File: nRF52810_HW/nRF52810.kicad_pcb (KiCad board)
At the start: 4 copper layers, 62.2 x 65.2 mm, 70 parts, among them J1 TC2050-IDC-NL, Q1 BSS138PW,115, U1 NRF52810-QCAA-R, U2 PMW3360DM-T2QU, U3 AP2114HA-3.3TRG1, U4 TPS61220DCKR, X1 XL7EL89CKI-111YLC-32M, X2 SC-20S32.768kHz20PPM9pF, X3 WJ500V-5.08-2P-14-00A

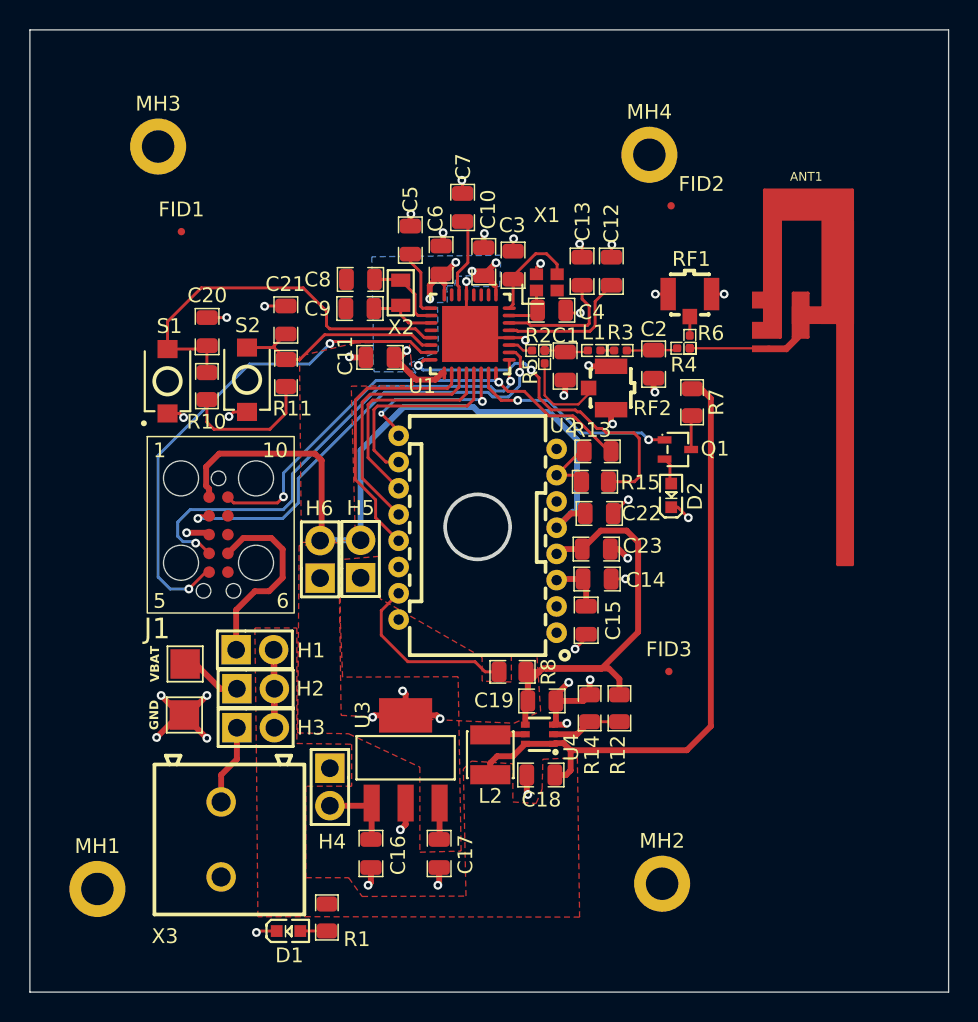
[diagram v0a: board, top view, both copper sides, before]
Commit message: Bulk change
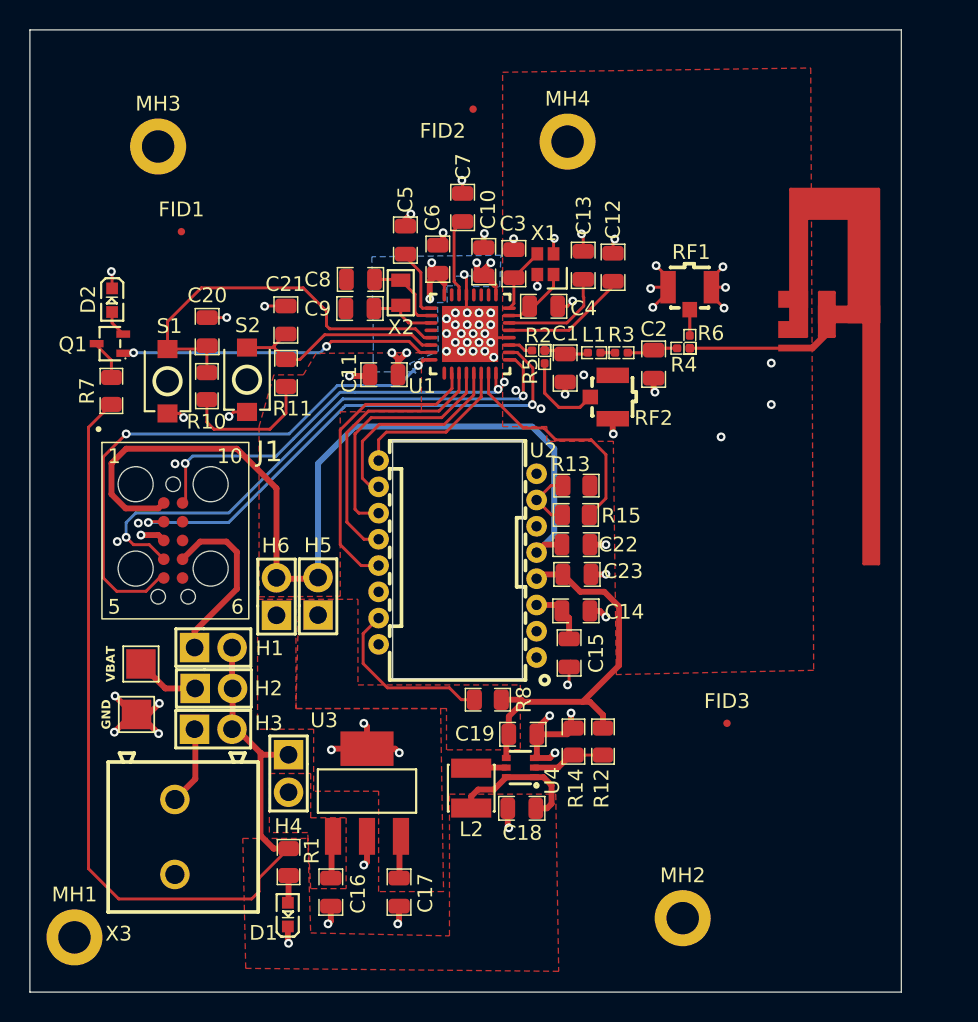
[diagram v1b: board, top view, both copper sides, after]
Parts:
- moved D2 40.2 mm to (45.5, 114.0), turned to 90 degrees
- moved R7 39.3 mm to (45.5, 120.1), turned to 90 degrees
- moved Q1 39.1 mm to (45.4, 116.9), turned to 0 degrees
- moved FID2 14.9 mm to (70.0, 101.0), turned to 180 degrees
- moved MH4 5.61 mm to (76.4, 103.2)
- moved FID3 5.28 mm to (87.2, 142.6)
- moved R1 4.56 mm to (57.5, 152.0)
- moved H6 3.89 mm to (56.7, 134.0)
- moved H5 3.83 mm to (59.5, 134.0)
- moved C16 3.77 mm to (60.4, 154.0)
- moved C17 3.77 mm to (65.0, 154.0)
- moved MH1 3.63 mm to (43.0, 157.1)
- moved U3 3.45 mm to (62.8, 147.3)
- moved ANT1 3.30 mm to (94.5, 116.4)
- moved TP2 3.24 mm to (47.2, 142.0)
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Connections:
- U1 pad 15: /LED -> /nRST_MAN
- U1 pad 7: /GEN -> /LED
- U1 pad 8: /nRST_MAN -> /GEN
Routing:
- net /VIN: track 54.1 -> 75.9 mm
- net /VDD_MCU: track 74.0 -> 83.8 mm, vias 5 -> 6
- net /nRST_MAN: track 24.0 -> 15.6 mm, vias 2 -> 0
- net /LED: track 14.4 -> 21.5 mm
- net /VDD_1.9V: track 33.6 -> 26.6 mm
- net GND: track 67.2 -> 73.7 mm, vias 43 -> 78
- net /nRESET: track 33.2 -> 27.2 mm
- net /SWDCLK: track 33.0 -> 37.7 mm
- net /SWDIO: track 30.4 -> 34.9 mm
- net /GEN: track 34.5 -> 38.0 mm
- net /VIN_LDO: track 5.39 -> 2.49 mm
- net /XC2: track 6.86 -> 4.47 mm
- net /nCS: track 18.5 -> 20.7 mm
- net /MISO: track 16.6 -> 18.7 mm
- net /MOSI: track 14.9 -> 16.9 mm
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- added copper zone on F.Cu, net /VIN_LDO
- added copper zone on F.Cu, net GND
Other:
- board size 62.2 x 65.2 mm -> 59 x 65.2 mm
- board text added: "4.1"
